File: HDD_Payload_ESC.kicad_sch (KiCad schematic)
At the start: 27 parts, among them J1 Conn_01x05_Pin, J2 Conn_01x03_Pin, J3 Conn_01x06_Pin, J4 Screw_Terminal_01x02, SW1 SW_Push, U1 STM32G431CBUx, U2 AP3402, Y1 Crystal_GND24

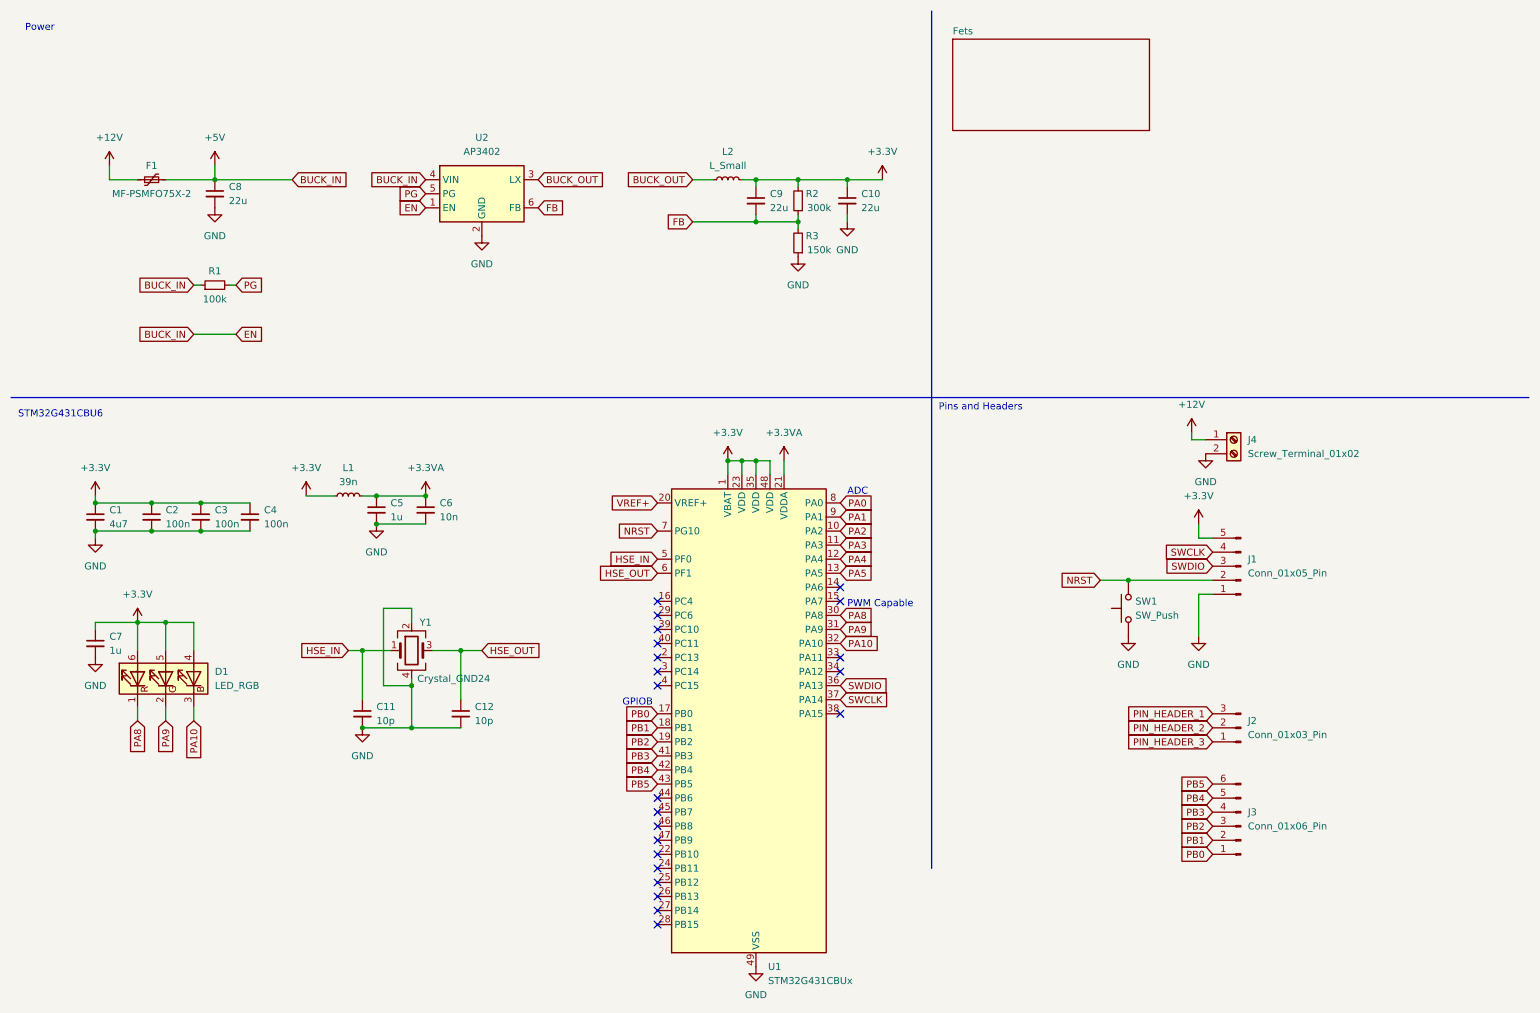
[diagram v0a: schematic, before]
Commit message: labeling update
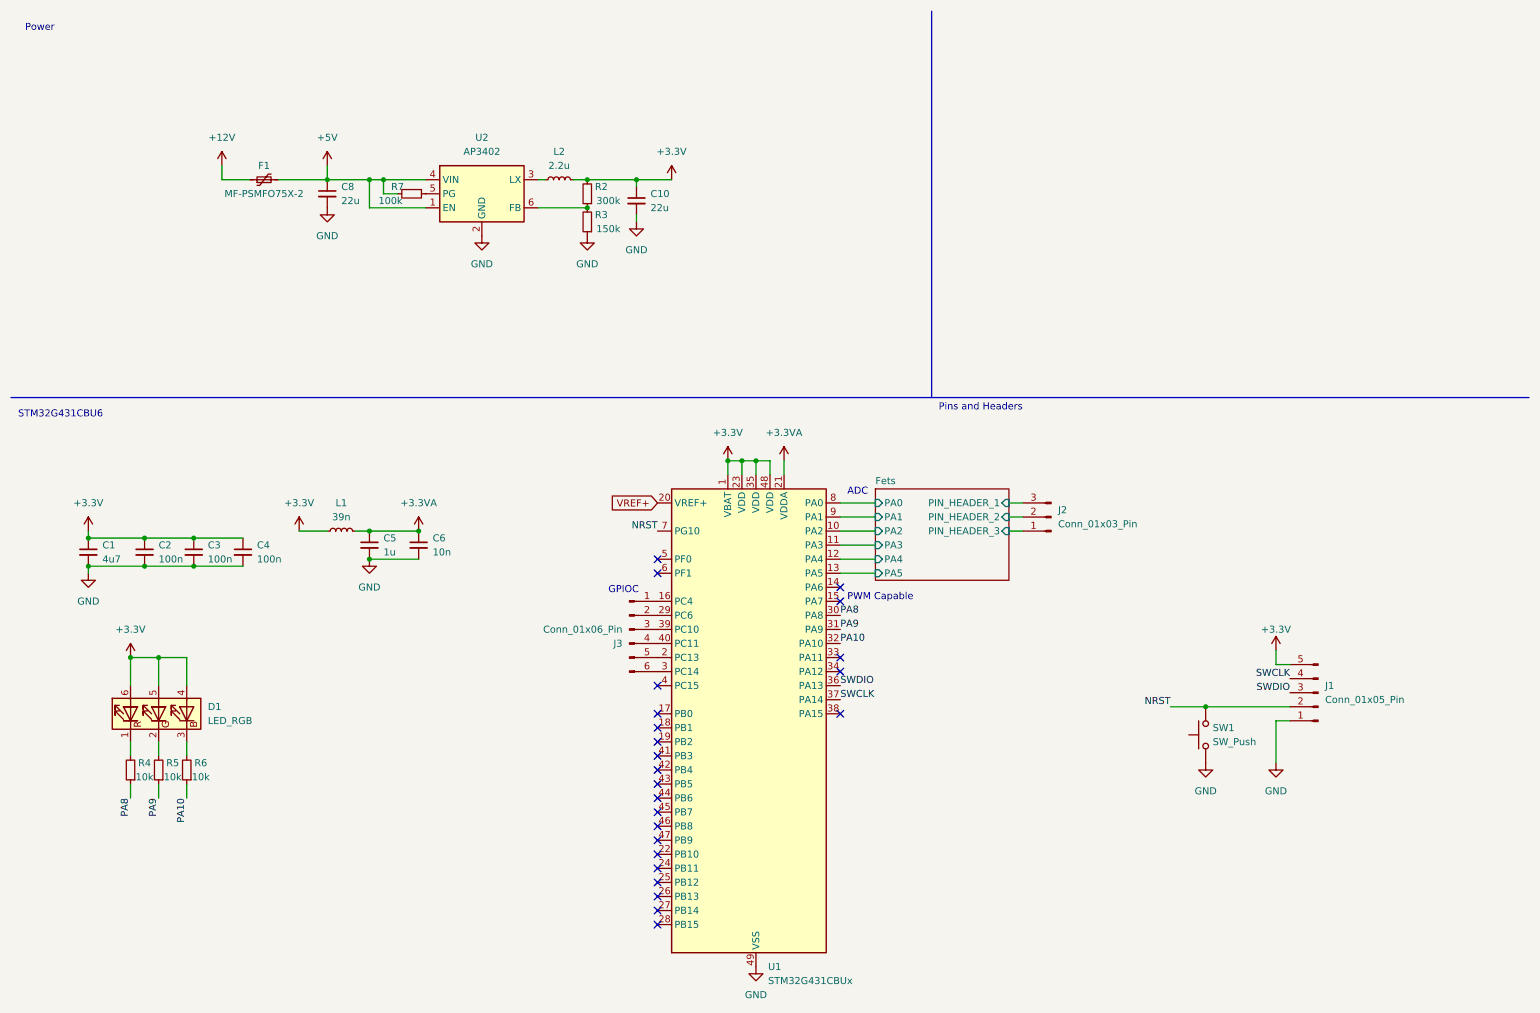
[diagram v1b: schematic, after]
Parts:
- removed C11, C12: 10p, Capacitor_SMD:C_0402_1005Metric, symbol Device:C_Small
- removed C7: 1u, Capacitor_SMD:C_0402_1005Metric, symbol Device:C_Small
- removed C9: 22u, symbol Device:C_Small
- removed J4: Screw_Terminal_01x02, symbol Connector:Screw_Terminal_01x02
- removed R1: 100k, symbol Device:R_Small
- removed Y1: Crystal_GND24, symbol Device:Crystal_GND24
- added R4, R5, R6: 10k, symbol Device:R_Small
- added R7: 100k, symbol Device:R_Small
- L2: value L_Small -> 2.2u
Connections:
- net +5V: now also R7.2
- net PA10: now also R6.1; no longer D1.3 (BK)
- net PA8: now also R4.1; no longer D1.1 (RK)
- net PA9: now also R5.1; no longer D1.2 (GK)
- net at U1.16 (PC4): now also J3.1 (Pin_1)
- net at U1.2 (PC13): now also J3.5 (Pin_5)
- net at U1.29 (PC6): now also J3.2 (Pin_2)
- net at U1.3 (PC14): now also J3.6 (Pin_6)
- net at U1.39 (PC10): now also J3.3 (Pin_3)
- net at U1.40 (PC11): now also J3.4 (Pin_4)
- net BUCK_OUT: no longer names the net of L2.1, U2.3 (LX)
- net FB: no longer names the net of R2.1, R3.2, U2.6 (FB)
- net HSE_IN: no longer names the net of U1.5 (PF0)
- net HSE_OUT: no longer names the net of U1.6 (PF1)
- net PA0 renamed Fets/PA0
- net PA1 renamed Fets/PA1
- net PA2 renamed Fets/PA2
- net PA3 renamed Fets/PA3
- net PA4 renamed Fets/PA4
- net PA5 renamed Fets/PA5
- net PB0: no longer names the net of U1.17 (PB0)
- net PB0: no longer J3.1 (Pin_1)
- net PB1: no longer names the net of U1.18 (PB1)
- net PB1: no longer J3.2 (Pin_2)
- net PB2: no longer names the net of U1.19 (PB2)
- net PB2: no longer J3.3 (Pin_3)
- net PB3: no longer names the net of U1.41 (PB3)
- net PB3: no longer J3.4 (Pin_4)
- net PB4: no longer names the net of U1.42 (PB4)
- net PB4: no longer J3.5 (Pin_5)
- net PB5: no longer names the net of U1.43 (PB5)
- net PB5: no longer J3.6 (Pin_6)
- net PG: no longer names the net of U2.5 (PG)
- net PG: now also R7.1
- net PIN_HEADER_1 renamed Fets/PIN_HEADER_1
- net PIN_HEADER_2 renamed Fets/PIN_HEADER_2
- net PIN_HEADER_3 renamed Fets/PIN_HEADER_3
- new net: D1.1 (RK), R4.2
- new net: D1.2 (GK), R5.2
- new net: D1.3 (BK), R6.2
- no-connect marks 22 -> 24
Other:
- sheet Fets ports: added PA0, PA1, PA2, PA3, PA4, PA5, PIN_HEADER_1, PIN_HEADER_2, PIN_HEADER_3; removed none
- note added: "GPIOC"
- note removed: "GPIOB"
- moved on the sheet: C1, C10, C2, C3, C4, C5, C6, C8, D1, F1, J1, J2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
